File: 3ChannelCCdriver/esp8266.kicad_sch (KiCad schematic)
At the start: 13 parts, among them J1 BB10-10S-02, U6 ESP-12F, U7 XC6210B332MR

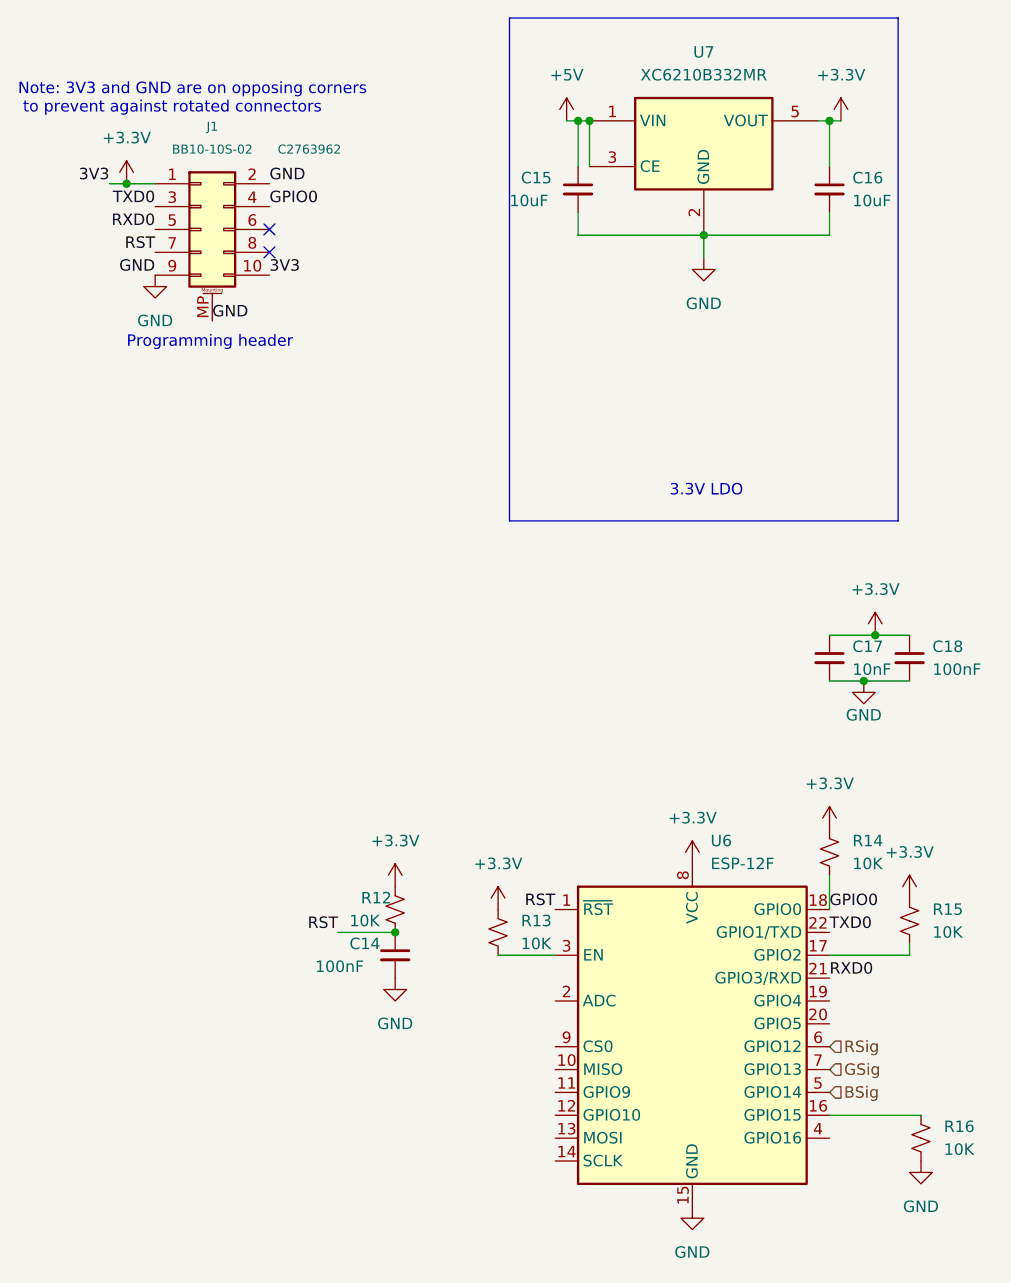
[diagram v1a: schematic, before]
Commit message: neat-ified schematics
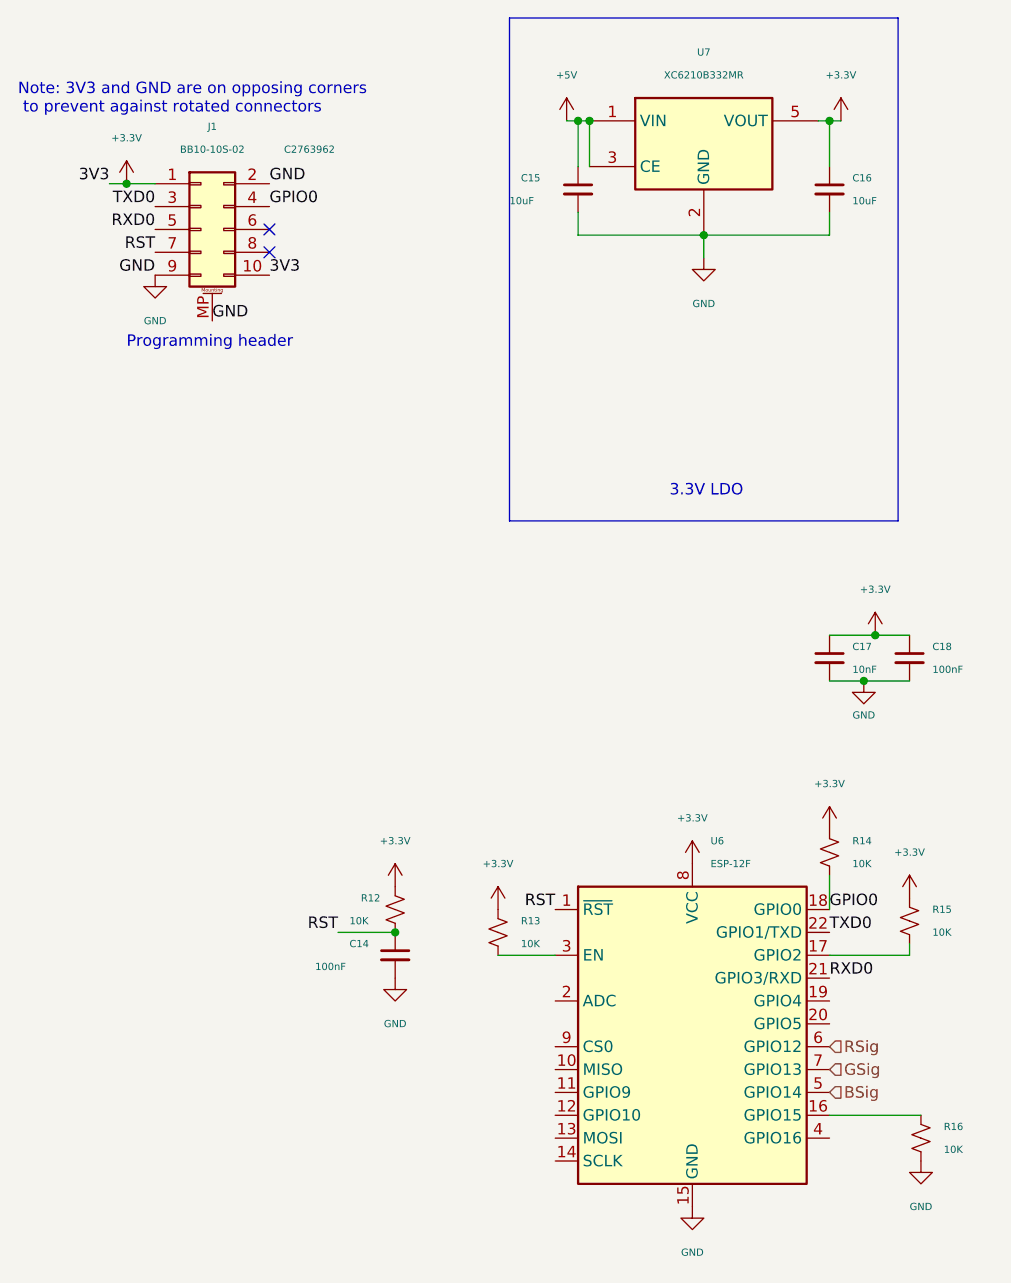
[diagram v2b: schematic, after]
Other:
- title: (none) -> ESP8266 MCU
